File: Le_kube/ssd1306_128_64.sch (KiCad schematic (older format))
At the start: 11 parts, among them U2 128x64_OLED

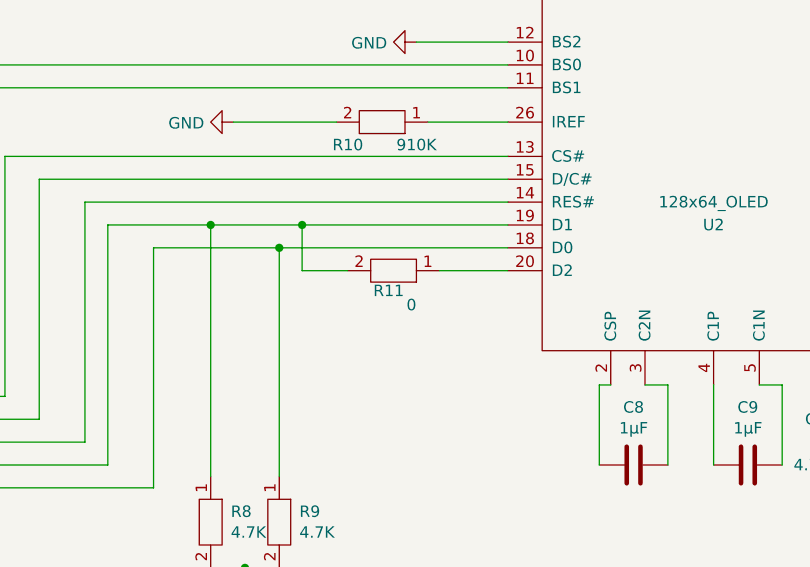
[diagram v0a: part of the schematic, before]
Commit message: corrections
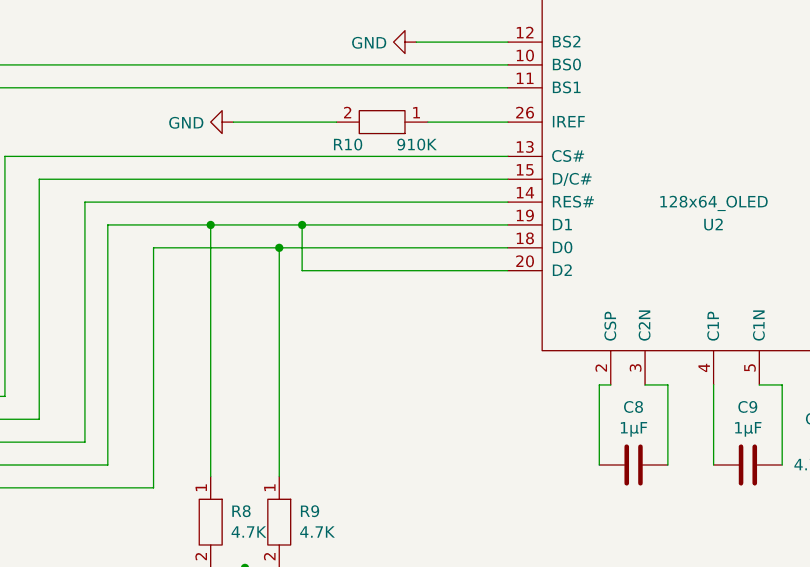
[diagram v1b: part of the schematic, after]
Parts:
- removed R11: 0, symbol Kube_library:R
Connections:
- net SDA_D1: now also U2.20 (D2)
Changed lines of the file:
@@
 	4050 3650 4050 2600
-Wire Wire Line
-	5600 2700 5300 2700
-$Comp
-L Kube_library:R R11
-U 1 1 60712FDF
-P 5100 2700
-F 0 "R11" H 5054 2788 50  0000 L CNN
-F 1 "0" H 5000 2850 50  0000 L CNN
-F 2 "" H 5100 2700 50  0001 C CNN
-F 3 "" H 5100 2700 50  0001 C CNN
-	1    5100 2700
-	-1   0    0    1
-$EndComp
-Wire Wire Line
-	4900 2700 4700 2700
 Wire Wire Line
 	4700 2700 4700 2500
@@
 	0    1    1    0
 $EndComp
+Wire Wire Line
+	4700 2700 5600 2700
 $EndSCHEMATC

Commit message: footprints done
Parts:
- C10, C11, C12, C13, C8, C9: footprint (none) -> Le_kube:C_0603_1608Metric_Pad1.08x0.95mm_HandSolder
- R10, R8, R9: footprint (none) -> Le_kube:R_0603_1608Metric_Pad0.98x0.95mm_HandSolder
- U2: footprint (none) -> Le_kube:OLED-0.96-12864
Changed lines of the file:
@@
 F 0 "R10" H 5200 2150 50  0000 C CNN
 F 1 "910K" H 4900 2150 50  0000 C CNN
-F 2 "" H 5050 2050 50  0001 C CNN
+F 2 "Le_kube:R_0603_1608Metric_Pad0.98x0.95mm_HandSolder" H 5050 2050 50  0001 C CNN
 F 3 "" H 5050 2050 50  0001 C CNN
 	1    5050 2050
@@
 F 0 "C8" H 6150 3802 50  0000 C CNN
 F 1 "1µF" H 6150 3711 50  0000 C CNN
-F 2 "" V 6300 3588 50  0001 C CNN
+F 2 "Le_kube:C_0603_1608Metric_Pad1.08x0.95mm_HandSolder" V 6300 3588 50  0001 C CNN
 F 3 "~" H 6150 3550 50  0001 C CNN
 	1    6150 3550
@@
 F 0 "C9" H 6650 3802 50  0000 C CNN
 F 1 "1µF" H 6650 3711 50  0000 C CNN
-F 2 "" V 6800 3588 50  0001 C CNN
+F 2 "Le_kube:C_0603_1608Metric_Pad1.08x0.95mm_HandSolder" V 6800 3588 50  0001 C CNN
 F 3 "~" H 6650 3550 50  0001 C CNN
 	1    6650 3550
@@
 F 0 "C10" V 7150 3600 50  0000 R CNN
 F 1 "4.7µF" V 6950 3650 50  0000 R CNN
-F 2 "" V 7200 3488 50  0001 C CNN
+F 2 "Le_kube:C_0603_1608Metric_Pad1.08x0.95mm_HandSolder" V 7200 3488 50  0001 C CNN
 F 3 "~" H 7050 3450 50  0001 C CNN
 	1    7050 3450
@@
 F 0 "C11" V 7350 3600 50  0000 R CNN
 F 1 "2.2µF" V 7150 3400 50  0000 R CNN
-F 2 "" V 7400 3488 50  0001 C CNN
+F 2 "Le_kube:C_0603_1608Metric_Pad1.08x0.95mm_HandSolder" V 7400 3488 50  0001 C CNN
 F 3 "~" H 7250 3450 50  0001 C CNN
 	1    7250 3450
@@
 F 0 "C12" V 8854 2915 50  0000 L CNN
 F 1 "1µF" V 8945 2915 50  0000 L CNN
-F 2 "" V 9050 2838 50  0001 C CNN
+F 2 "Le_kube:C_0603_1608Metric_Pad1.08x0.95mm_HandSolder" V 9050 2838 50  0001 C CNN
 F 3 "~" H 8900 2800 50  0001 C CNN
 	1    8900 2800
@@
 F 0 "C13" V 9254 2915 50  0000 L CNN
 F 1 "1µF" V 9345 2915 50  0000 L CNN
-F 2 "" V 9450 2838 50  0001 C CNN
+F 2 "Le_kube:C_0603_1608Metric_Pad1.08x0.95mm_HandSolder" V 9450 2838 50  0001 C CNN
 F 3 "~" H 9300 2800 50  0001 C CNN
 	1    9300 2800
@@
 F 0 "U2" H 6500 2500 50  0000 C CNN
 F 1 "128x64_OLED" H 6500 2600 50  0000 C CNN
-F 2 "" H 6750 2500 50  0001 C CNN
+F 2 "Le_kube:OLED-0.96-12864" H 6750 2500 50  0001 C CNN
 F 3 "~" H 6750 2500 50  0001 C CNN
 	1    6750 2500
@@
 F 0 "R9" V 4554 3888 50  0000 L CNN
 F 1 "4.7K" V 4645 3888 50  0000 L CNN
-F 2 "" H 4600 3800 50  0001 C CNN
+F 2 "Le_kube:R_0603_1608Metric_Pad0.98x0.95mm_HandSolder" H 4600 3800 50  0001 C CNN
 F 3 "" H 4600 3800 50  0001 C CNN
 	1    4600 3800
@@
 F 0 "R8" V 4254 3888 50  0000 L CNN
 F 1 "4.7K" V 4345 3888 50  0000 L CNN
-F 2 "" H 4300 3800 50  0001 C CNN
+F 2 "Le_kube:R_0603_1608Metric_Pad0.98x0.95mm_HandSolder" H 4300 3800 50  0001 C CNN
 F 3 "" H 4300 3800 50  0001 C CNN
 	1    4300 3800
